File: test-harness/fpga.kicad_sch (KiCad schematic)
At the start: 33 parts, among them J2 Conn_ARM_JTAG_SWD_10, J3 Conn_01x16, J4 Conn_01x16, J5 Conn_01x06, U1 MachXO3D_9400

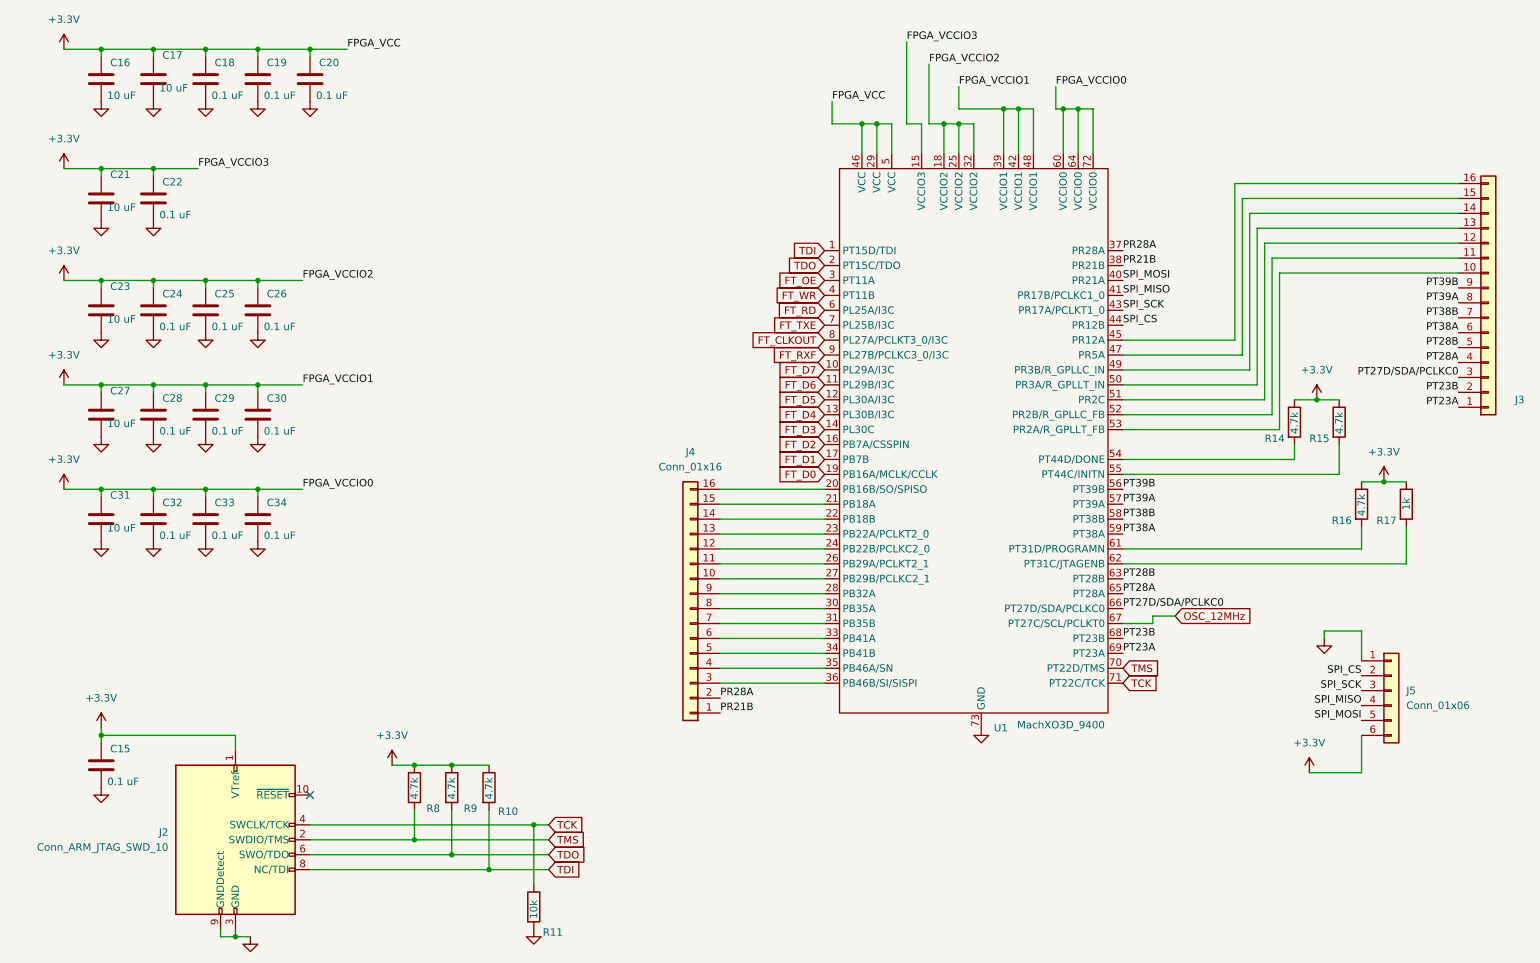
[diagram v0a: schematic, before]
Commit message: Test harness v2
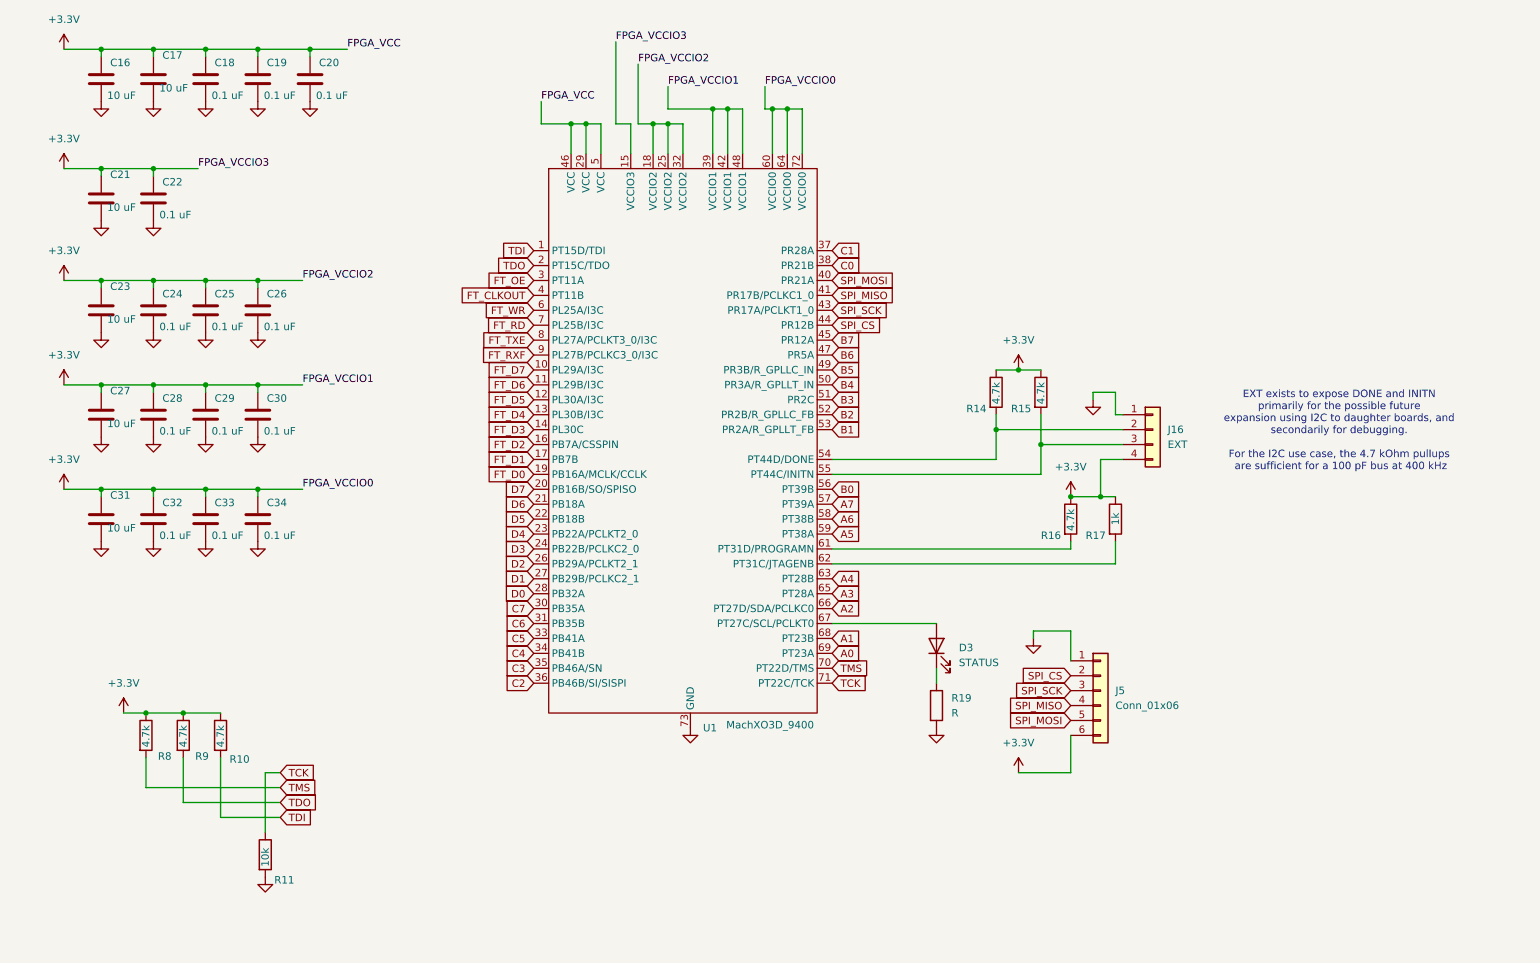
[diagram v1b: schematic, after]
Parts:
- removed C15: 0.1 uF, Capacitor_SMD:C_0805_2012Metric, symbol Device:C
- removed J2: Conn_ARM_JTAG_SWD_10, Connector_PinHeader_1.27mm:PinHeader_2x05_P1.27mm_Vertical_SMD, symbol Connector:Conn_ARM_JTAG_SWD_10
- removed J3, J4: Conn_01x16, Connector_PinHeader_2.54mm:PinHeader_1x16_P2.54mm_Vertical, symbol Connector_Generic:Conn_01x16
- added D3: STATUS, LED_SMD:LED_0805_2012Metric, symbol Device:LED
- added J16: EXT, Connector_PinHeader_2.54mm:PinHeader_1x04_P2.54mm_Vertical, symbol Connector_Generic:Conn_01x04
- added R19: R, Resistor_SMD:R_0805_2012Metric, symbol Device:R
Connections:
- net +3.3V: now also J16.4 (Pin_4)
- net FT_CLKOUT: now also U1.4 (PT11B); no longer U1.8 (PL27A/PCLKT3_0/I3C)
- net FT_RD: now also U1.7 (PL25B/I3C); no longer U1.6 (PL25A/I3C)
- net FT_TXE: now also U1.8 (PL27A/PCLKT3_0/I3C); no longer U1.7 (PL25B/I3C)
- net FT_WR: now also U1.6 (PL25A/I3C); no longer U1.4 (PT11B)
- net GND: now also J16.1 (Pin_1), R19.2
- net at R15.2, U1.55 (PT44C/INITN): now also J16.3 (Pin_3)
- net D1: now reaches U1.27 (PB29B/PCLKC2_1)
- net D2: now reaches U1.26 (PB29A/PCLKT2_1)
- net D3: now reaches U1.24 (PB22B/PCLKC2_0)
- net D4: now reaches U1.23 (PB22A/PCLKT2_0)
- net D5: now reaches U1.22 (PB18B)
- net D6: now reaches U1.21 (PB18A)
- net D7: now reaches U1.20 (PB16B/SO/SPISO)
- net C2: now reaches U1.36 (PB46B/SI/SISPI)
- net C3: now reaches U1.35 (PB46A/SN)
- net C4: now reaches U1.34 (PB41B)
- net C5: now reaches U1.33 (PB41A)
- net C6: now reaches U1.31 (PB35B)
- net C7: now reaches U1.30 (PB35A)
- net D0: now reaches U1.28 (PB32A)
- net B7: now reaches U1.45 (PR12A)
- net B6: now reaches U1.47 (PR5A)
- net B5: now reaches U1.49 (PR3B/R_GPLLC_IN)
- net B4: now reaches U1.50 (PR3A/R_GPLLT_IN)
- net B3: now reaches U1.51 (PR2C)
- net B2: now reaches U1.52 (PR2B/R_GPLLC_FB)
- net B1: now reaches U1.53 (PR2A/R_GPLLT_FB)
- net at R14.2, U1.54 (PT44D/DONE): now also J16.2 (Pin_2)
- net OSC_12MHz: no longer names the net of U1.67 (PT27C/SCL/PCLKT0)
- net OSC_12MHz: now also D3.2 (A)
- net PR21B renamed C0
- net PR28A renamed C1
- net PT23A renamed A0
- net PT23B renamed A1
- net PT27D/SDA/PCLKC0 renamed A2
- net PT28A renamed A3
- net PT28B renamed A4
- net PT38A renamed A5
- net PT38B renamed A6
- net PT39A renamed A7
- net PT39B renamed B0
- new net: D3.1 (K), R19.1
- no-connect marks 1 -> 0
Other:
- note added: "EXT exists to expose DONE and INITN primarily for the possible future expansion using I2C to daughter boards, and secondarily for debugging. For the I2C use case, the 4.7 kOhm pullups are sufficient for a 100 pF bus at 400 kHz"
- moved on the sheet: J5, R10, R11, R14, R15, R16, R17, R8, R9, U1
